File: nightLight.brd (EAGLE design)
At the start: 46.6 x 55.9 mm, 18 parts, among them Q1 200mA/40V

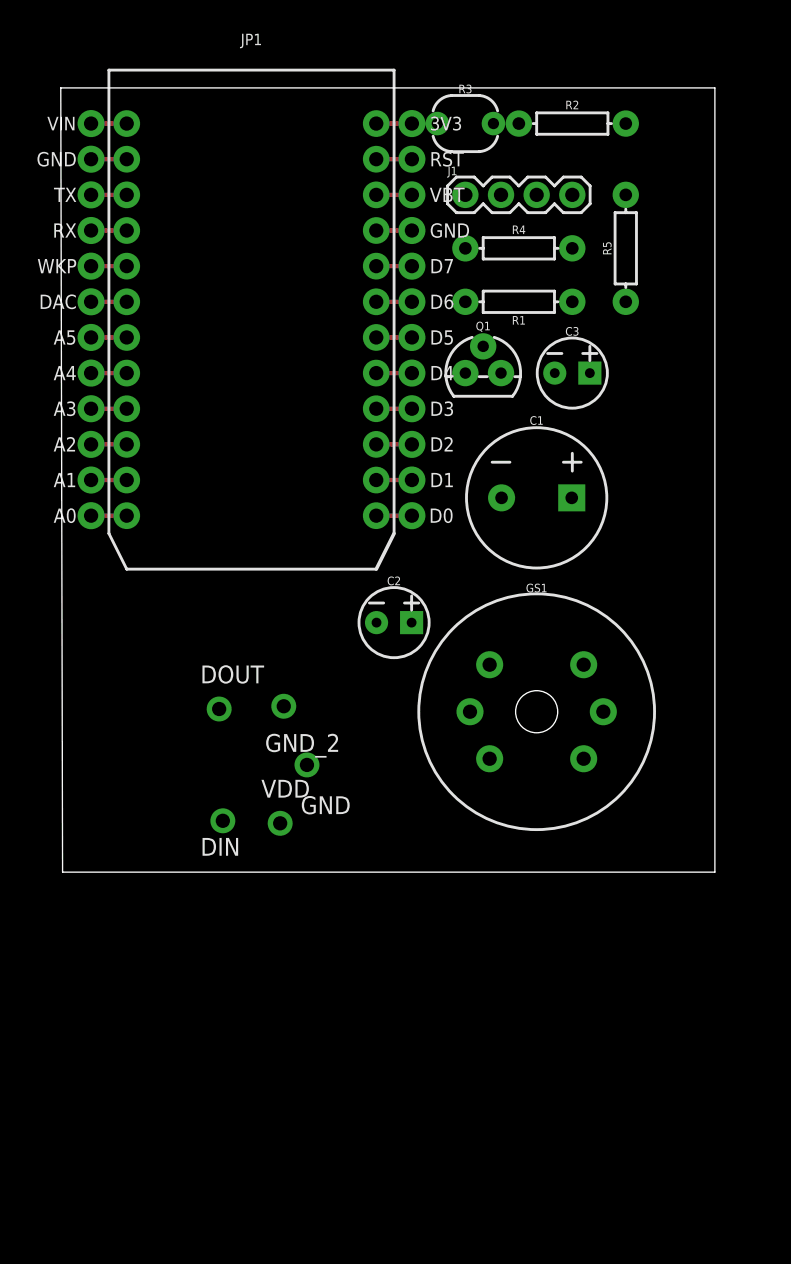
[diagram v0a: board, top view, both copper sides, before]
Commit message: This is the board i ordered
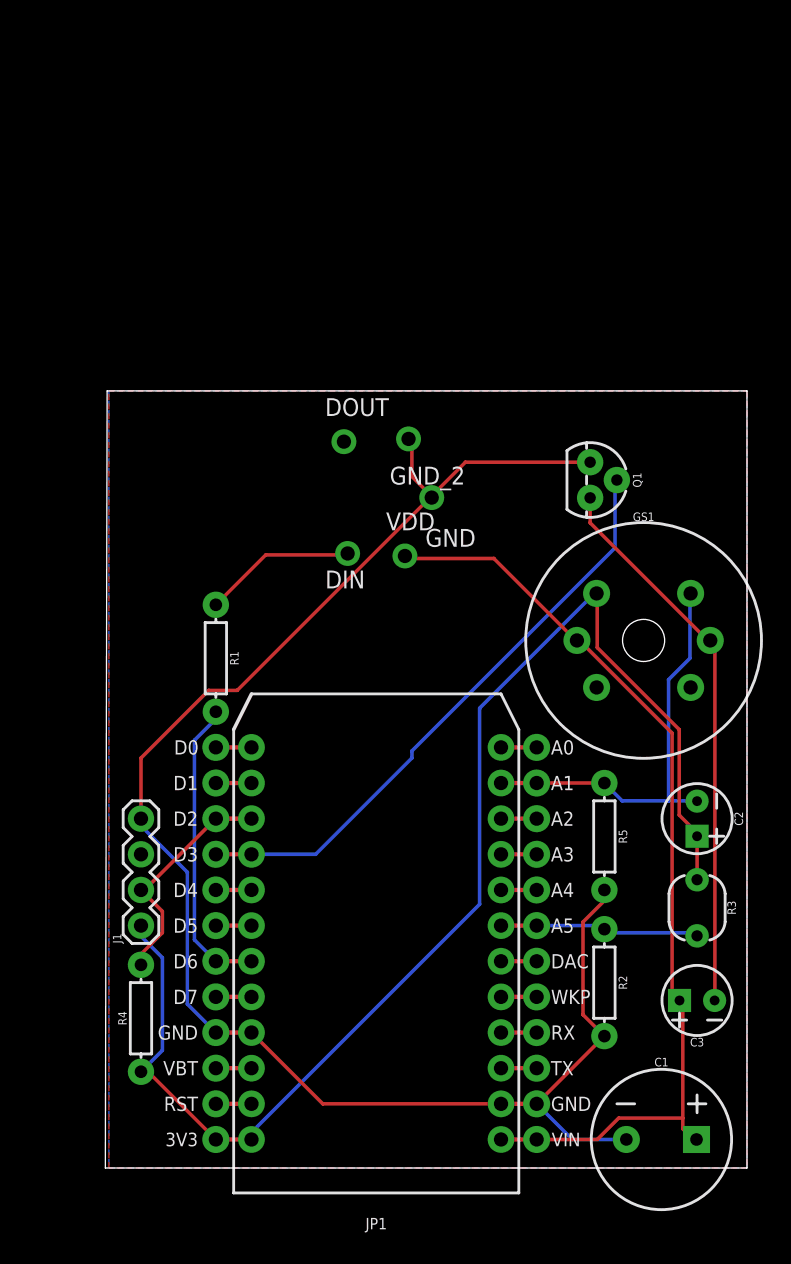
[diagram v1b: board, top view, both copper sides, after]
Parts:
- removed FRAME1: FRAME-LETTER, SparkFun-Aesthetics:CREATIVE_COMMONS
- moved R2 61.3 mm to (40.4, 16.3), turned to 270 degrees
- moved R4 61.1 mm to (7.37, 13.7), turned to 90 degrees
- moved R3 58.3 mm to (47.0, 21.6), turned to 270 degrees
- moved J1 57.0 mm to (7.37, 20.3), turned to 90 degrees
- moved JP1 47.8 mm to (24.1, 17.8), turned to 180 degrees
- moved C1 46.6 mm to (44.5, 5.08)
- moved C3 45.6 mm to (47.0, 15.0), turned to 180 degrees
- moved R5 41.9 mm to (40.4, 26.7), turned to 270 degrees
- moved R1 33.3 mm to (12.7, 39.4), turned to 270 degrees
- moved C2 25.7 mm to (47.0, 27.9), turned to 270 degrees
- moved GND 21.0 mm to (28.1, 50.8)
- moved VDD 21.0 mm to (26.2, 46.7)
- moved DIN 21.0 mm to (22.1, 46.8)
- moved DOUT 21.0 mm to (21.8, 54.8)
- moved GND_2 21.0 mm to (26.4, 55.0)
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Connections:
- new net A5: JP1.7, JP1.A5, R2.P$1, R3.2
- net A0: no longer R2.P$1, R3.2
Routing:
- net GND: track 3.09 -> 118.3 mm
- net 3V3: track 1.13 -> 91.5 mm
- net 5V: track 0.11 -> 65.2 mm
- net D3: track 0.00 -> 40.2 mm
- net N$2: track 0.00 -> 39.7 mm
- net A1: track 0.00 -> 27.4 mm
- net D6: track 0.10 -> 21.6 mm
- net D2: track 1.47 -> 16.6 mm
- net A5: track 0.00 -> 11.9 mm
- net N$1: track 0.00 -> 10.9 mm
- net VBAT: track 0.10 -> 2.54 mm
- added copper zone on layer 1, net GND
- added copper zone on layer 16, net GND
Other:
- board size 46.6 x 55.9 mm -> 45.7 x 55.4 mm
